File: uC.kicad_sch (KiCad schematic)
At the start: 18 parts, among them J1 Conn_02x03_ESP_PROG, J11 GPIO Conn, J12 UEXT_Host, J2 I2C Conn, J4 MCU head, U2 ESP32-S3-WROOM-1

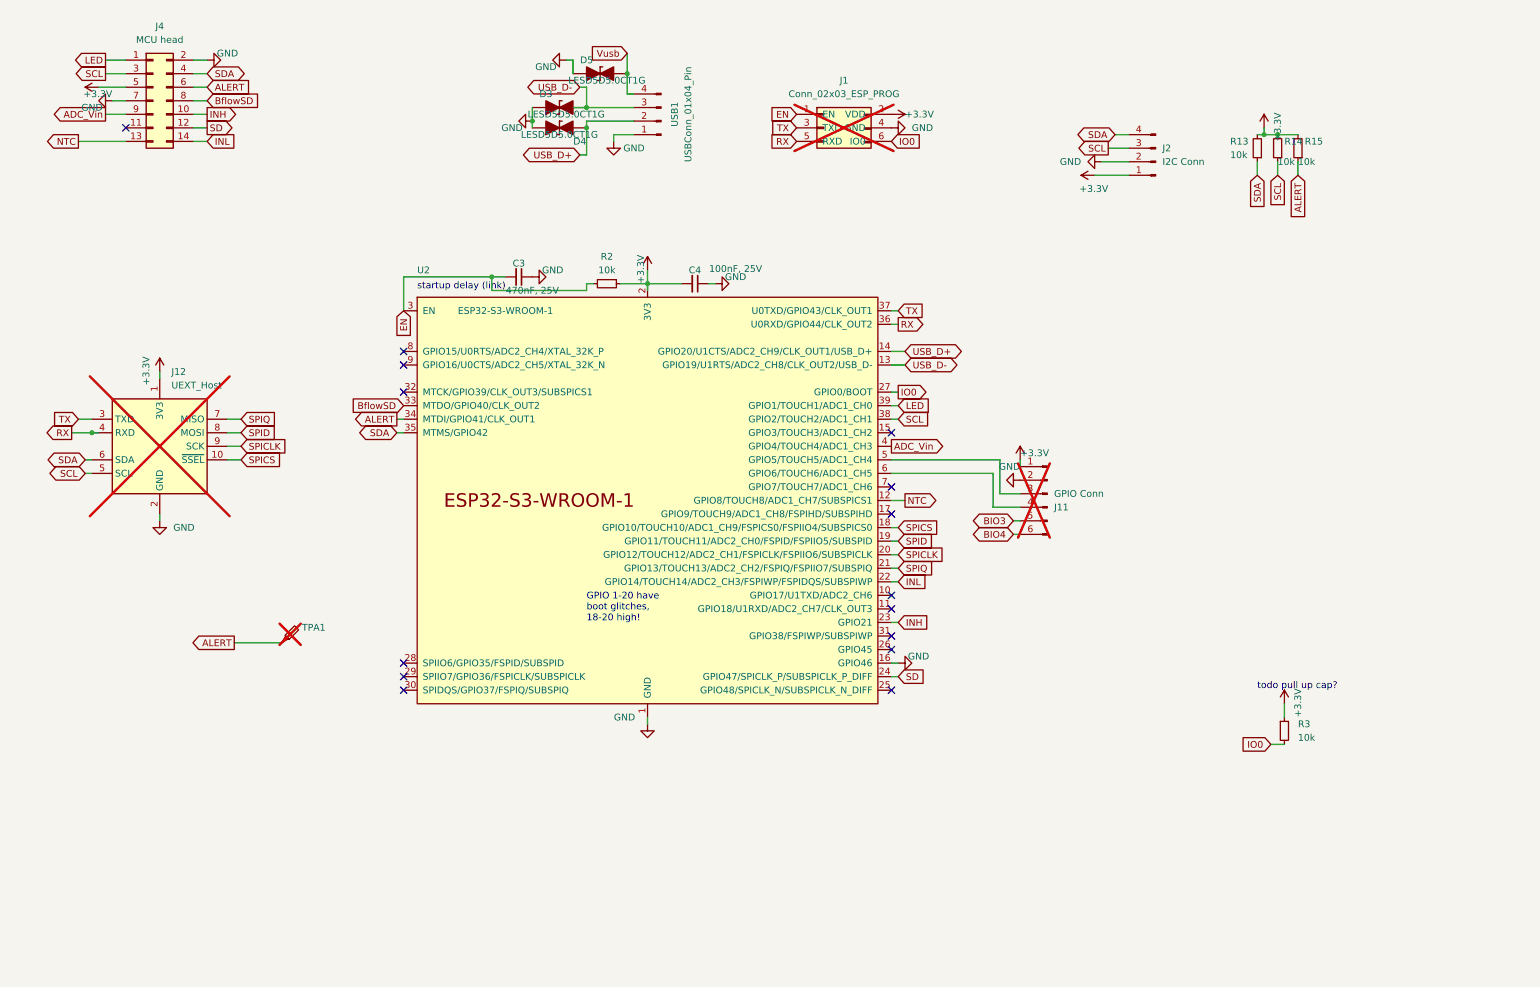
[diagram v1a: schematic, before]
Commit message: First cut, with refactored schematic (PCB now busted, it's a WIP)
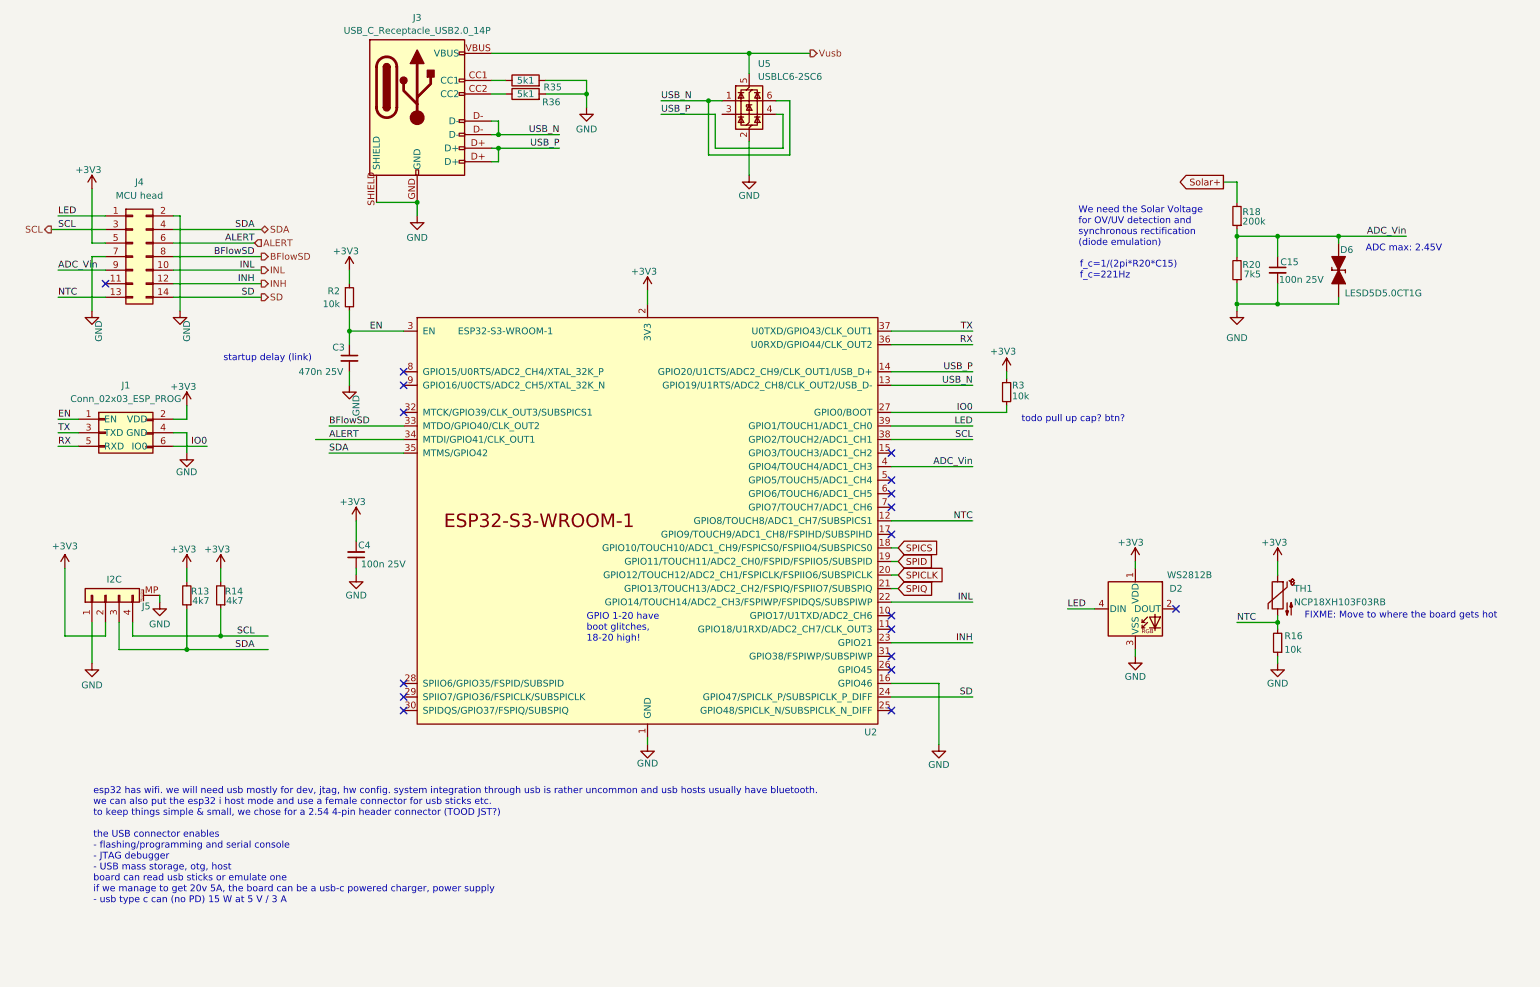
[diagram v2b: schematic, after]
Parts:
- removed D3, D4, D5: LESD5D5.0CT1G, Diode_SMD:D_SOD-523, symbol PCM_Diode_TVS_AKL:D_TVS_Bidirectional_Generic
- removed J11: GPIO Conn, Connector_PinHeader_1.27mm:PinHeader_1x06_P1.27mm_Vertical, symbol Connector:Conn_01x06_Pin
- removed J12: UEXT_Host, Connector_PinHeader_2.54mm:PinHeader_2x05_P2.54mm_Vertical_SMD, symbol Connector:UEXT_Host
- removed J2: I2C Conn, Connector_PinSocket_2.00mm:PinSocket_1x04_P2.00mm_Vertical, symbol Connector:Conn_01x04_Pin
- removed R15: 10k, Resistor_SMD:R_0805_2012Metric, symbol Device:R_Small
- removed TPA1: ~, TestPoint:TestPoint_Pad_D1.0mm, symbol Connector:TestPoint_Probe
- removed USB1: USBConn_01x04_Pin, Connector_PinHeader_2.54mm:PinHeader_1x04_P2.54mm_Vertical, symbol Connector:Conn_01x04_Pin
- added C15: 100n 25V, Capacitor_SMD:C_0805_2012Metric, symbol Device:C_Small
- added D2: WS2812B, LED_SMD:LED_WS2812B_PLCC4_5.0x5.0mm_P3.2mm, symbol LED:WS2812B
- added D6: LESD5D5.0CT1G, Diode_SMD:D_SOD-523, symbol PCM_Diode_TVS_AKL:D_TVS_Bidirectional_Generic
- added J3: USB_C_Receptacle_USB2.0_14P, afork-kicad-parts:USB-C-SMD_G-SWITCH_GT-USB-7010ASV, symbol afork-kicad-parts:USB_C_Receptacle_USB2.0_14P
- added J5: I2C, Connector_JST:JST_SH_SM04B-SRSS-TB_1x04-1MP_P1.00mm_Horizontal, symbol Connector_Generic_MountingPin:Conn_01x04_MountingPin
- added R16: 10k, Resistor_SMD:R_0805_2012Metric, symbol Device:R_Small
- added R18: 200k, Resistor_SMD:R_0805_2012Metric, symbol Device:R_Small
- added R20: 7k5, Resistor_SMD:R_0805_2012Metric, symbol Device:R_Small
- added R35, R36: 5k1, Resistor_SMD:R_0805_2012Metric, symbol Device:R
- added TH1: NCP18XH103F03RB, Resistor_SMD:R_0603_1608Metric_Pad0.98x0.95mm_HandSolder, symbol Device:Thermistor_NTC
- added U5: USBLC6-2SC6, Package_TO_SOT_SMD:SOT-23-6, symbol Power_Protection:USBLC6-2SC6
- C3: value 470nF, 25V -> 470n 25V
- C4: value 100nF, 25V -> 100n 25V
- J1: now fitted; now in the parts list
- R13, R14: value 10k -> 4k7
- U2: footprint open-pe:ESP32-S3-WROOM-1-noPIN15 -> RF_Module:ESP32-S3-WROOM-1
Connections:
- net ADC_Vin: now also C15.1, D6.1 (K), R18.1, R20.2
- net EN: now also C3.1; no longer C3.2
- net GND: now also C3.2, C15.2, D2.3 (VSS), D6.2 (A), J3.GND, J3.SHIELD, J5.1 (Pin_1), J5.MP (MountPin), R16.1, R20.1, R35.2, R36.2, U5.2 (GND); no longer C3.1
- net INH: now also J4.12 (Pin_12); no longer J4.10 (Pin_10)
- net INL: now also J4.10 (Pin_10); no longer J4.14 (Pin_14)
- net LED: now also D2.4 (DIN)
- net NTC: now also R16.2, TH1.2
- net SCL: now also J5.4 (Pin_4)
- net SD: now also J4.14 (Pin_14); no longer J4.12 (Pin_12)
- net SDA: now also J5.3 (Pin_3)
- net Vusb: now also J3.VBUS, U5.5 (VBUS)
- net +3.3V renamed +3V3
- net +3V3: now also D2.1 (VDD), J5.2 (Pin_2), TH1.1
- net BflowSD renamed BFlowSD
- net USB_D+ renamed USB_P
- net USB_P: now also J3.D+, U5.4 (I/O2)
- net USB_D- renamed USB_N
- net USB_N: now also J3.D-, U5.1 (I/O1), U5.6 (I/O1)
- new net: J3.CC1, R35.1
- new net: J3.CC2, R36.1
- new net Solar+: R18.2
- no-connect marks 15 -> 18
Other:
- note added: "ADC max: 2.45V"
- note added: "FIXME: Move to where the board gets hot"
- note added: "We need the Solar Voltage for OV/UV detection and synchronous rectification (diode emulation)"
- note added: "esp32 has wifi. we will need usb mostly for dev, jtag, hw config. system integration through usb is rather uncommon and usb hosts usually have bluetooth. we can also put the esp32 i host mode and use a female connector for usb sticks etc. to keep things simple & small, we chose for a 2.54 4-pin header connector (TOOD JST?) the USB connector enables - flashing/programming and serial console - JTAG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"
- note added: "f_c=1/(2pi*R20*C15) f_c=221Hz"
- note added: "todo pull up cap? btn?"
- note removed: "todo pull up cap?"
- moved on the sheet: C3, C4, J4, R13, R14, R2, R3, U2

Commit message: Mega-cleanup
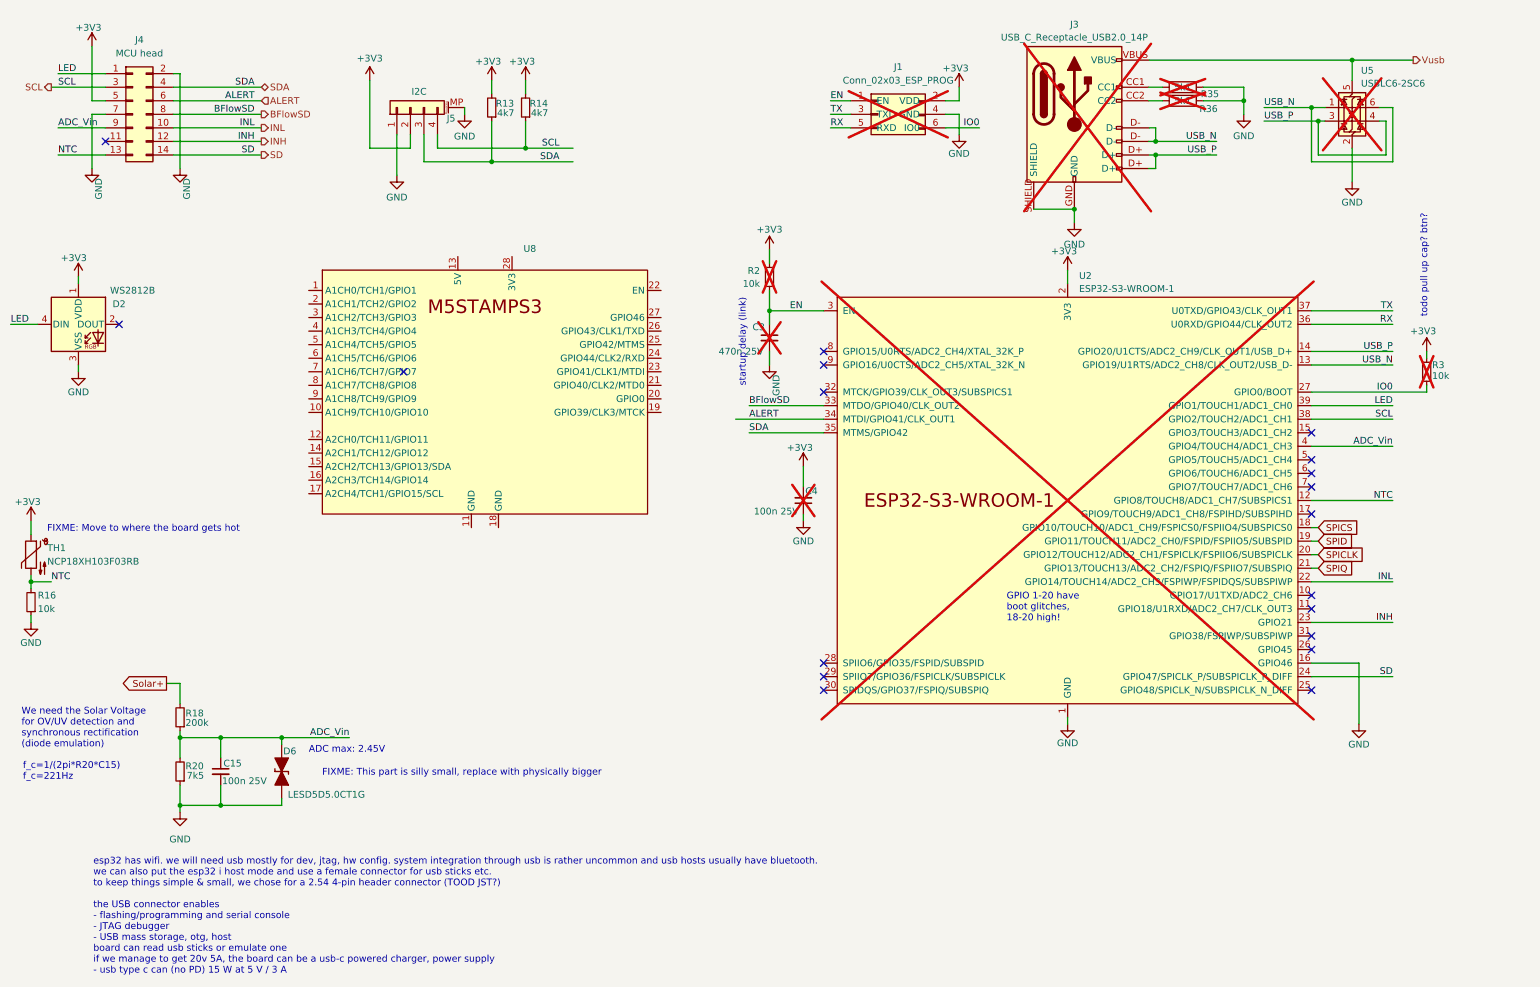
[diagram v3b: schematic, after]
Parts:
- added U8: ~, afork-kicad-parts:STAMP-S3-DIP, symbol afork-kicad-parts:M5STAMPS3
- C3, C4, J1, J3, R2, R3, R35, R36, U2, U5: now not fitted
- D6: LCSC (none) -> C5199850
- J4: footprint open-pe:PinHeader_2x07_P2.54mm_Vertical_SMD_Pin1Left -> Connector_PinHeader_2.54mm:PinHeader_2x07_P2.54mm_Vertical
- J5: footprint Connector_JST:JST_SH_SM04B-SRSS-TB_1x04-1MP_P1.00mm_Horizontal -> afork-kicad-parts:JST_SH_SM04B-SRSS-TB_1x04-1MP_P1.00mm_Horizontal; TODO 1 -> (none)
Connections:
- net USB_P: now also U5.3 (I/O2)
- no-connect marks 18 -> 19
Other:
- note added: "FIXME: This part is silly small, replace with physically bigger"
- moved on the sheet: C15, D2, D6, J4, J5, R13, R14, R16, R18, R20, TH1
